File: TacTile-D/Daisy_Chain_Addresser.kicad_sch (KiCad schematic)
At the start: 7 parts, among them U1 74LS04, U16 74LS74, U2 4011, U6 74HC08, U7 74LS74, U8 4042, U9 74HC4051

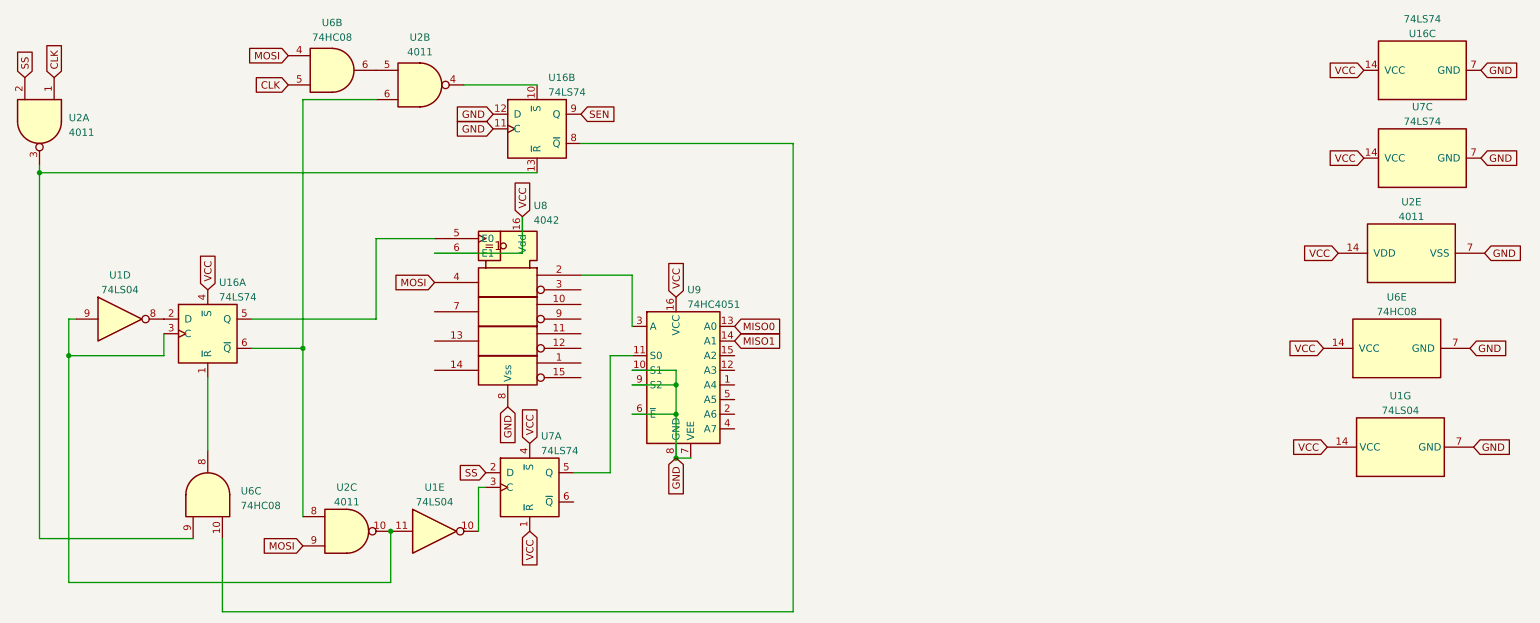
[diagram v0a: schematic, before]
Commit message: Fixed issues with D board and rerouted
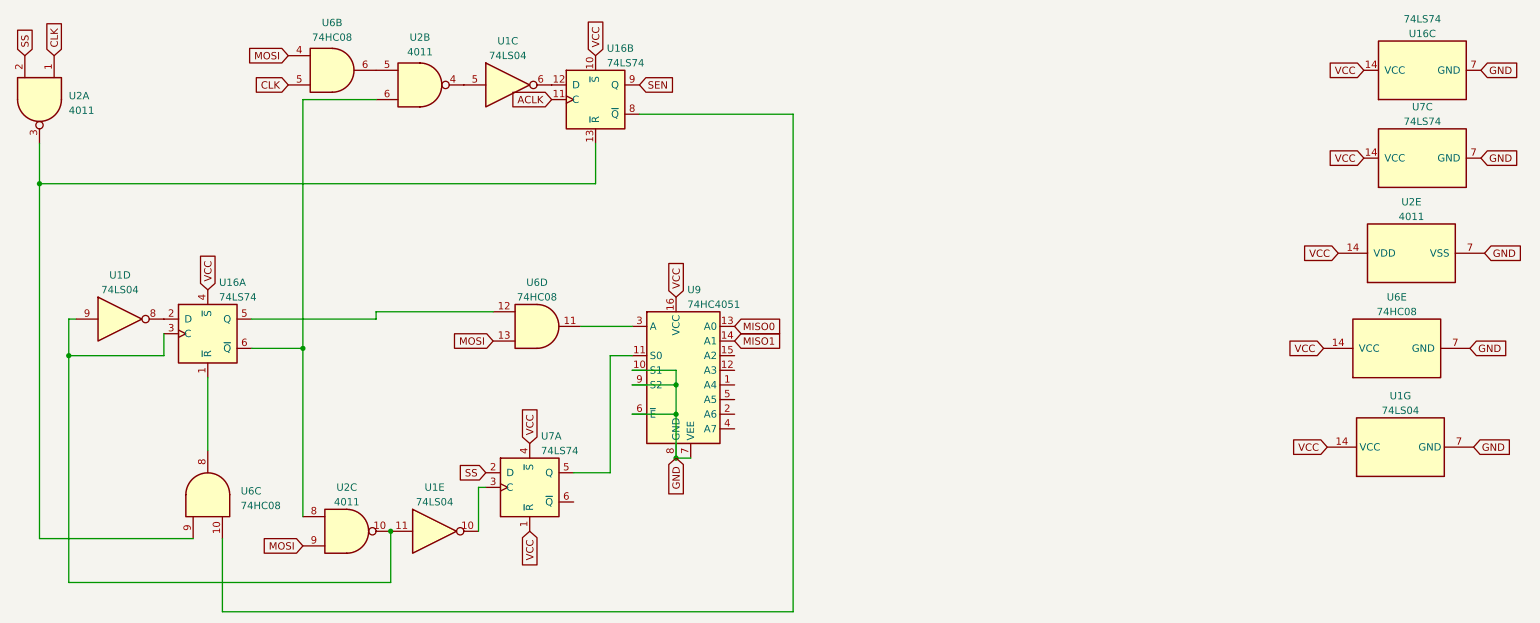
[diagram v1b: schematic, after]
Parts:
- removed U8: 4042, Package_DIP:DIP-16_W7.62mm, symbol 4xxx_IEEE:4042
- added unit 3 of U1
- added unit 4 of U6
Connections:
- net GND: no longer U16.11 (C), U16.12 (D)
- net MOSI: now also U6.13
- net VCC: now also U16.10 (~{S})
- net at U16.5 (Q): now also U6.12
- net at U2.4: now also U1.5; no longer U16.10 (~{S})
- net at U9.3 (A): now also U6.11
- new net: U1.6, U16.12 (D)
- new net ACLK: U16.11 (C)
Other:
- moved on the sheet: U16B, U2A
